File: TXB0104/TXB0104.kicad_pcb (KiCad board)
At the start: 2 copper layers, 13 x 15.5 mm, 8 parts, among them J1 Conn_01x06, J2 Conn_01x06

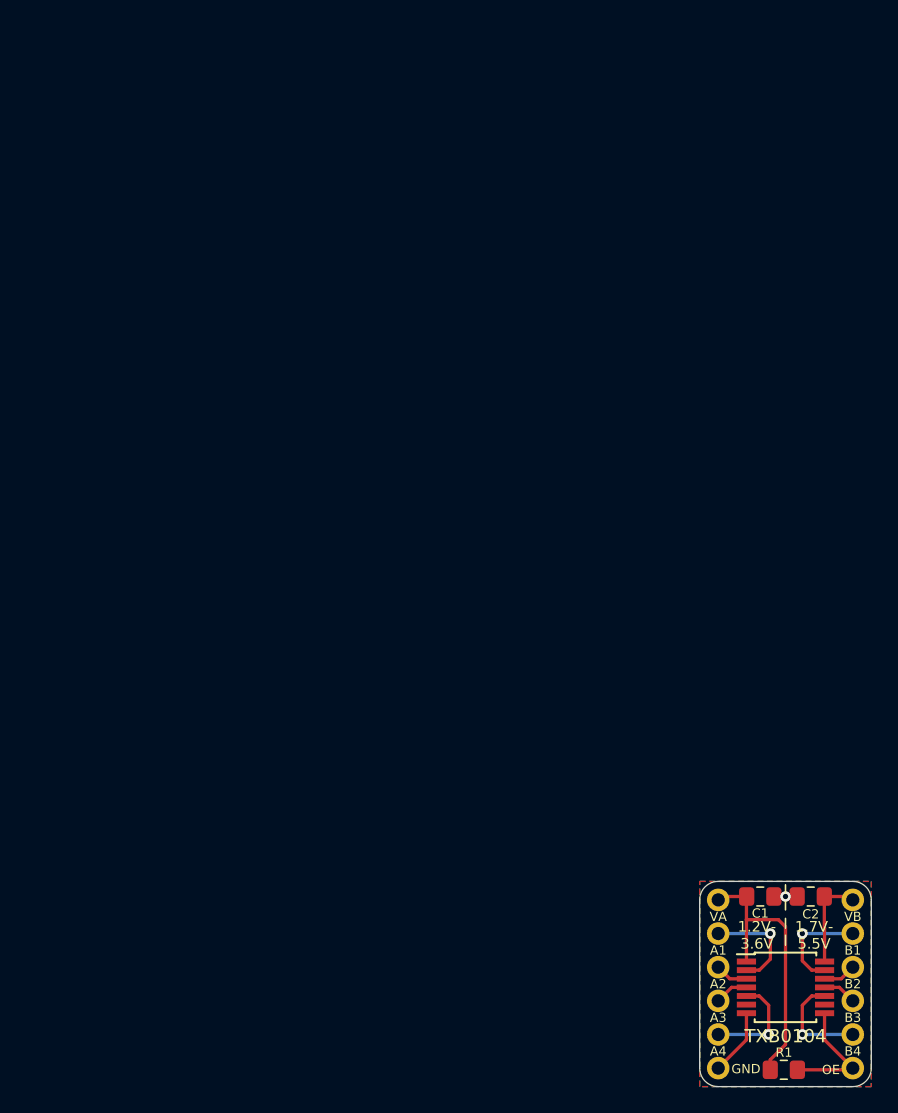
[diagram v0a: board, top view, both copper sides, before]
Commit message: Part Numbers Added
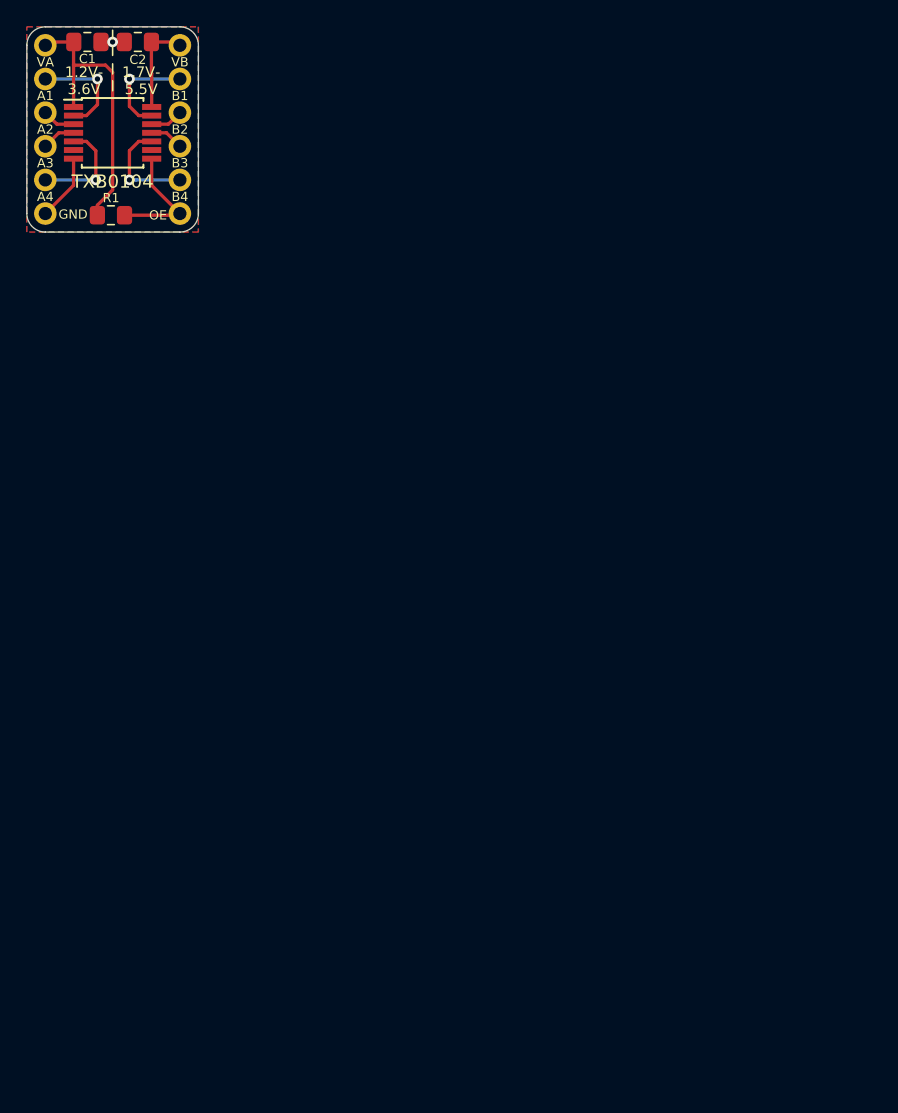
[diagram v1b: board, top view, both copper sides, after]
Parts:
- moved J2 82.1 mm to (71.4, 34.0)
- moved C1 82.1 mm to (64.4, 33.8)
- moved C2 82.1 mm to (68.2, 33.8)
- moved G*** 82.1 mm to (66.3, 34.9)
- moved J1 82.1 mm to (61.2, 34.0)
- moved R1 82.1 mm to (66.2, 46.9)
- moved TXB0104 82.1 mm to (66.3, 40.6)
- moved G*** 82.1 mm to (66.3, 38.2)
